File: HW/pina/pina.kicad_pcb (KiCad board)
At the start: 2 copper layers, 52 parts, among them U1 SN74LXC8T245PW, U2 LM2575-5.0BU, U3 INA228, U4 INA228

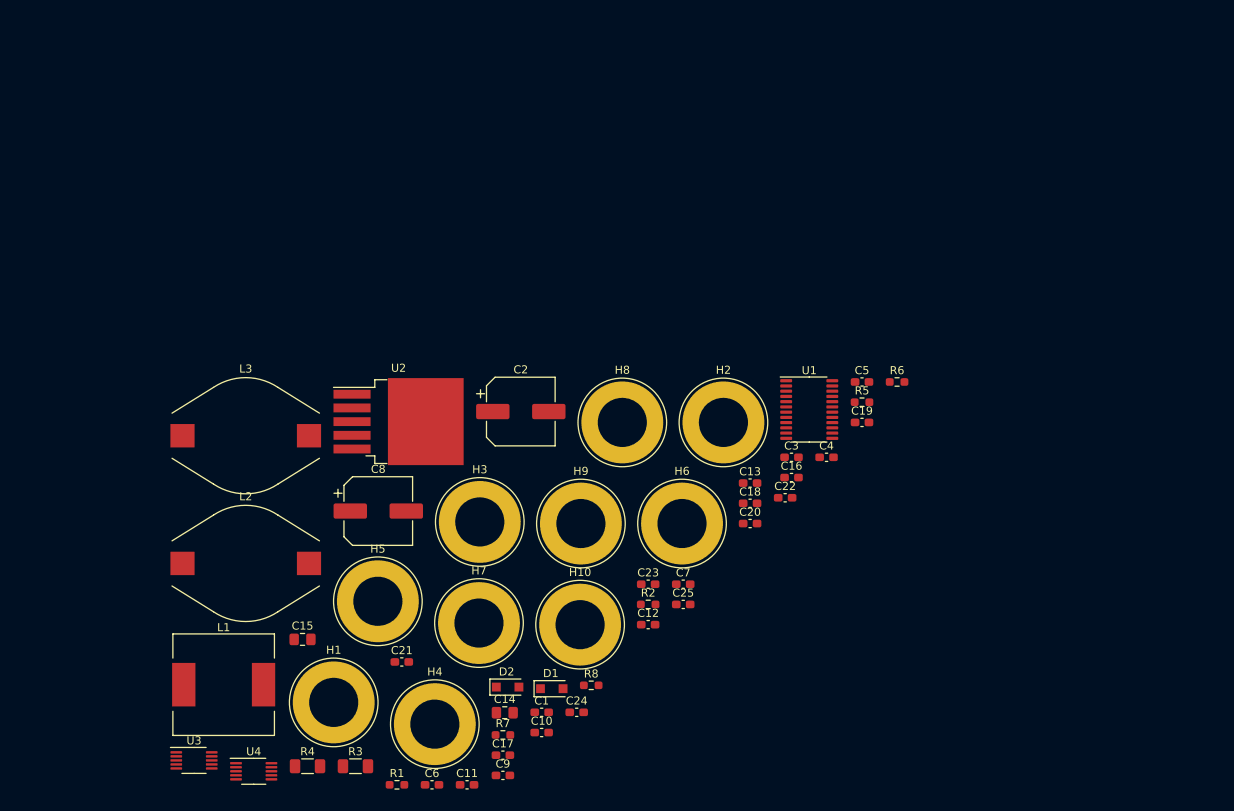
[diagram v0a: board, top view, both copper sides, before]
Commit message: Initial pcb added
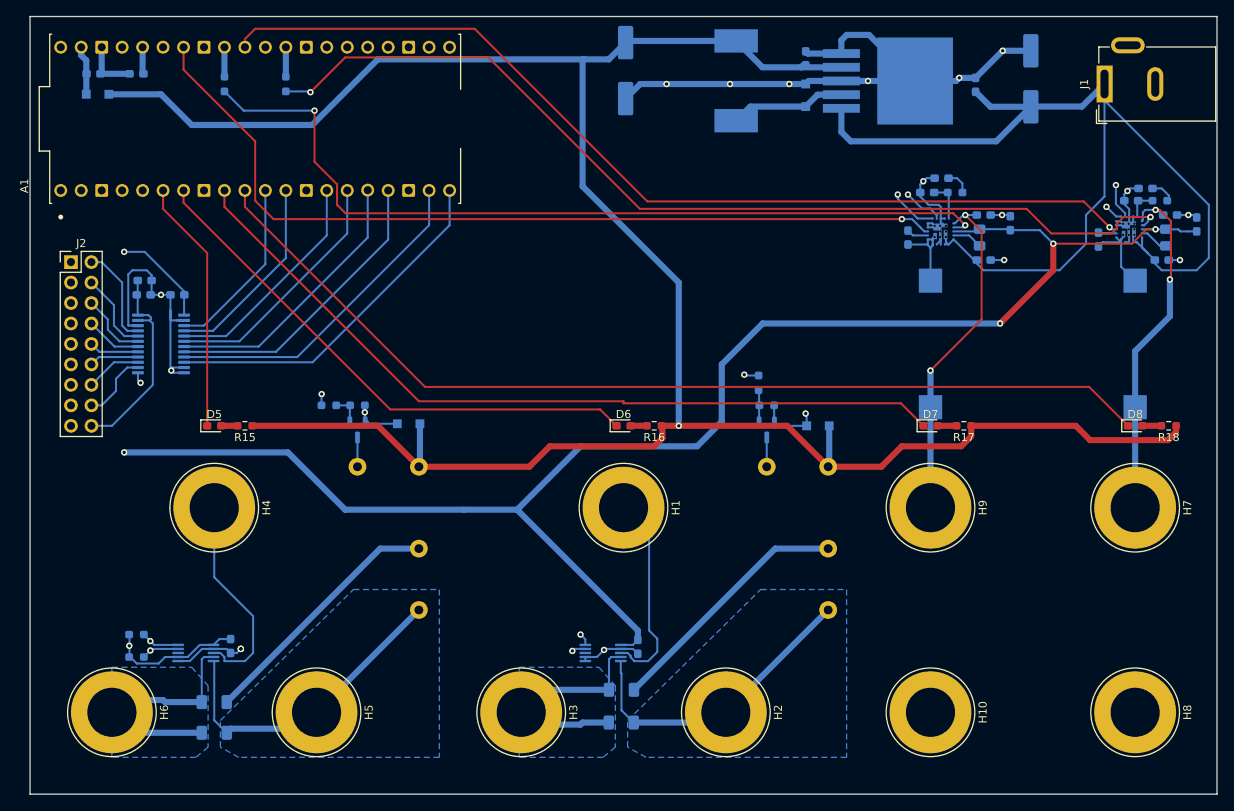
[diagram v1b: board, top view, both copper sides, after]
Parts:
- added A1: SC0918, g6b:MODULE_SC0918, F.Cu at (113.3, 53.6)
- added D3: 1N5819, Diode_SMD:D_SOD-123F, B.Cu at (183.1, 91.7)
- added D4: 1N5819, Diode_SMD:D_SOD-123F, B.Cu at (132.3, 91.4)
- added D5: LED, LED_SMD:LED_0603_1608Metric_Pad1.05x0.95mm_HandSolder, F.Cu at (108.2, 91.7)
- added D6: LED, LED_SMD:LED_0603_1608Metric_Pad1.05x0.95mm_HandSolder, F.Cu at (159.0, 91.7)
- added D7: LED, LED_SMD:LED_0603_1608Metric_Pad1.05x0.95mm_HandSolder, F.Cu at (197.1, 91.7)
- added D8: LED, LED_SMD:LED_0603_1608Metric_Pad1.05x0.95mm_HandSolder, F.Cu at (222.5, 91.7)
- added J1: 12V-DC, Connector_BarrelJack:BarrelJack_GCT_DCJ200-10-A_Horizontal, F.Cu at (218.7, 49.3)
- added J2: LogicInputs, Connector_PinHeader_2.54mm:PinHeader_2x09_P2.54mm_Vertical, F.Cu at (90.4, 71.4)
- added K1: G6B-1114P-US-DC5, g6b:RELAY_G6B_1114, B.Cu at (176.8, 96.8)
- added K2: G6B-1114P-US-DC5, g6b:RELAY_G6B_1114, B.Cu at (126.0, 96.8)
- added Q1: BSS138, Package_TO_SOT_SMD:SOT-23, B.Cu at (176.8, 92.2)
- added Q2: BSS138, Package_TO_SOT_SMD:SOT-23, B.Cu at (126.0, 92.2)
- added R10: 2K2, Resistor_SMD:R_0603_1608Metric_Pad0.98x0.95mm_HandSolder, B.Cu at (176.8, 89.2)
- added R11: 0.1, Resistor_SMD:R_1206_3216Metric_Pad1.30x1.75mm_HandSolder, B.Cu at (158.8, 124.5)
- added R12: 100, Resistor_SMD:R_0603_1608Metric_Pad0.98x0.95mm_HandSolder, B.Cu at (122.4, 89.2)
- added R13: 2K2, Resistor_SMD:R_0603_1608Metric_Pad0.98x0.95mm_HandSolder, B.Cu at (126.0, 89.2)
- added R14: 0.1, Resistor_SMD:R_1206_3216Metric_Pad1.30x1.75mm_HandSolder, B.Cu at (108.2, 126.0)
- added R15: 1K, Resistor_SMD:R_0603_1608Metric_Pad0.98x0.95mm_HandSolder, F.Cu at (112.0, 91.7)
- added R16: 1K, Resistor_SMD:R_0603_1608Metric_Pad0.98x0.95mm_HandSolder, F.Cu at (162.8, 91.7)
- added R17: 1K, Resistor_SMD:R_0603_1608Metric_Pad0.98x0.95mm_HandSolder, F.Cu at (201.2, 91.7)
- added R18: 1K, Resistor_SMD:R_0603_1608Metric_Pad0.98x0.95mm_HandSolder, F.Cu at (226.7, 91.7)
- added R9: 100, Resistor_SMD:R_0603_1608Metric_Pad0.98x0.95mm_HandSolder, B.Cu at (175.8, 86.4)
- added U5: MIC24045-EIYFL-TR, g6b:CONV_MIC24045-EIYFL-TR, B.Cu at (221.8, 67.3)
- added U6: MIC24045-EIYFL-TR, g6b:CONV_MIC24045-EIYFL-TR, B.Cu at (198.4, 67.6)
- C1, C10, C11, C12, C13, C14, C15, C16, C17, C18, C19, C2, C20, C21, C22, C23, C24, C25, C3, C4, C5, C6, C7, C8, C9, D1, D2, L1, L2, L3, R1, R2, R5, R6, R7, R8, U1, U2, U3, U4: moved to B.Cu
- R3, R4: value 0.1 -> 1; moved to B.Cu
- moved C6 117.7 mm to (230.1, 66.7), turned to 90 degrees
- moved L2 113.7 mm to (222.5, 81.5), turned to -90 degrees
- moved R7 105.1 mm to (225.6, 63.8)
- moved C14 101.0 mm to (226.3, 68.3), turned to 90 degrees
- moved L1 98.3 mm to (173.0, 48.9), turned to 90 degrees
- moved C15 97.7 mm to (203.2, 68.3), turned to 90 degrees
- moved C11 97.3 mm to (98.6, 48.0), turned to 180 degrees
- moved C7 96.8 mm to (93.2, 48.0)
- moved C9 96.6 mm to (181.6, 46.1), turned to 90 degrees
- moved D1 92.8 mm to (93.7, 50.5)
- moved R6 91.3 mm to (109.5, 49.3), turned to -90 degrees
- moved C21 91.1 mm to (203.7, 65.5), turned to 180 degrees
- moved C17 87.5 mm to (196.7, 62.7), turned to 180 degrees
- moved C4 87.4 mm to (99.6, 73.7)
- moved L3 85.7 mm to (197.1, 81.5), turned to -90 degrees
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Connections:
- net Net-(H2-Pad1) renamed /R_SH_1_P
- net Net-(H3-Pad1) renamed /R_SH_1_N
- net Net-(H5-Pad1) renamed /R_SH_2_P
- net Net-(H6-Pad1) renamed /R_SH_2_N
- U1 pad 14: /D7 -> /D0
- U1 pad 15: /D6 -> /D1
- U1 pad 16: /D5 -> /D2
- U1 pad 17: /D4 -> /D3
- U1 pad 18: /D3 -> /D4
- U1 pad 19: /D2 -> /D5
- U1 pad 2: unconnected-(U1-Pad2) -> GND
- U1 pad 20: /D1 -> /D6
- U1 pad 21: /D0 -> /D7
- U1 pad 22: unconnected-(U1-Pad22) -> GND
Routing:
- net /SDA: track 0.00 -> 343.4 mm, vias 0 -> 4
- net /SCL: track 0.00 -> 332.5 mm, vias 0 -> 4
- net +3V3: track 0.00 -> 328.0 mm, vias 0 -> 6
- net +5V: track 0.00 -> 286.6 mm, vias 0 -> 1
- net GND: track 0.00 -> 177.9 mm, vias 0 -> 20
- net +12V: track 0.00 -> 131.3 mm
- net /LED4: track 0.00 -> 122.9 mm
- net Net-(R5-Pad2): track 0.00 -> 121.2 mm, vias 0 -> 2
- net /PS1_PG: track 0.00 -> 120.0 mm, vias 0 -> 1
- net /PS2_PG: track 0.00 -> 107.8 mm, vias 0 -> 1
- net Net-(R6-Pad2): track 0.00 -> 105.6 mm, vias 0 -> 2
- net /LED3: track 0.00 -> 100.2 mm
- net /S1_ACT: track 0.00 -> 76.0 mm, vias 0 -> 1
- net /LED2: track 0.00 -> 66.7 mm
- net /S2_ACT: track 0.00 -> 52.9 mm, vias 0 -> 1
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- added copper zone on B.Cu, net /R_SH_1_N
- added copper zone on B.Cu, net /R_SH_1_P
- added copper zone on B.Cu, net /R_SH_2_N
- added copper zone on B.Cu, net /R_SH_2_P
- added copper zone on In1.Cu, net GND
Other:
- board outline added: 147.3 x 96.5 mm
- copper layers 2 -> 4
